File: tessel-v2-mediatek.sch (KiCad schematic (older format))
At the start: 46 parts, among them P201 CONN_01X02, U201 MT7620N, X201 20MHz

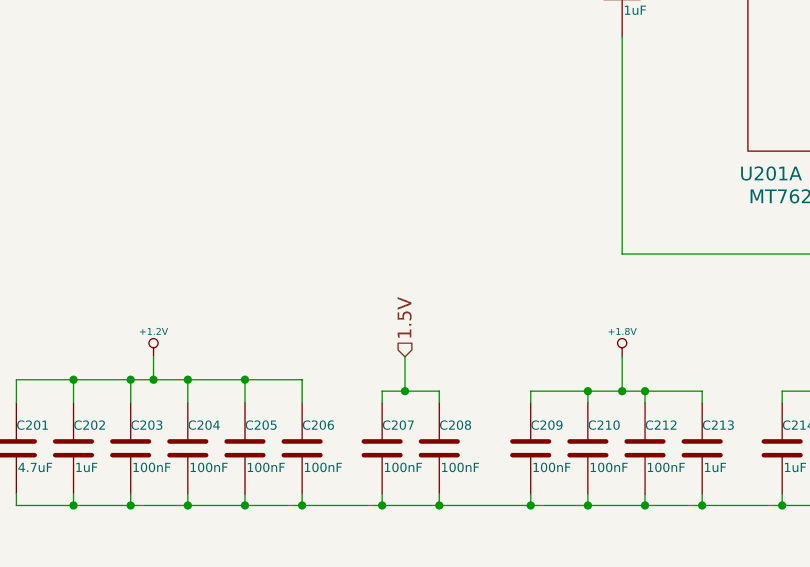
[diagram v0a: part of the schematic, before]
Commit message: second pass schem check
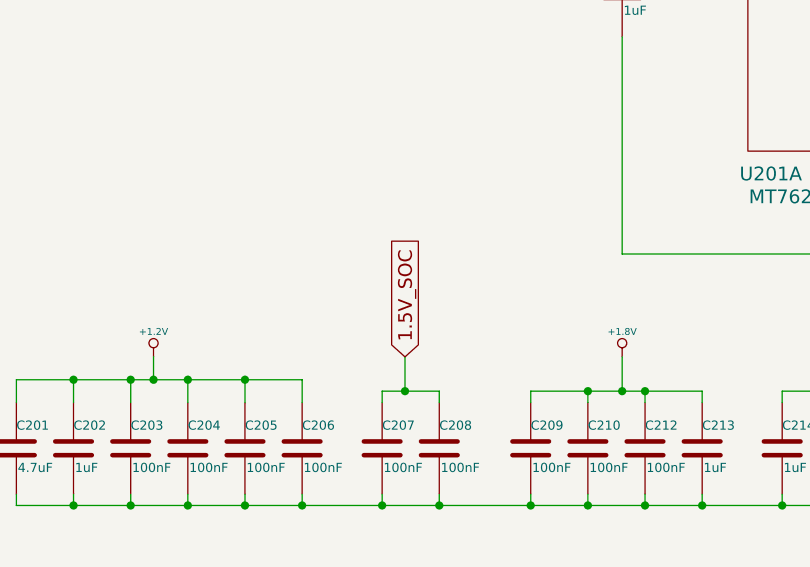
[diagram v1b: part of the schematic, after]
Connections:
- net 1.5V is gone; now on net 1.5V_SOC: C207.1, C208.1
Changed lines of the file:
@@
 	1    0    0    -1
 $EndComp
-Text HLabel 3850 8200 1    60   Input ~ 0
-1.5V
 $Comp
 L +1.2V #PWR205
@@
 Text GLabel 10550 5100 1    60   Input ~ 0
 1.5V_SOC
+Text GLabel 3850 8200 1    60   Input ~ 0
+1.5V_SOC
 $EndSCHEMATC
